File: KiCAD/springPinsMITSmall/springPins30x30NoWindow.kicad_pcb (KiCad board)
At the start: 2 copper layers, 30 x 30 mm, 22 parts, among them J1 CONN_02X06, J2 CONN_02X06

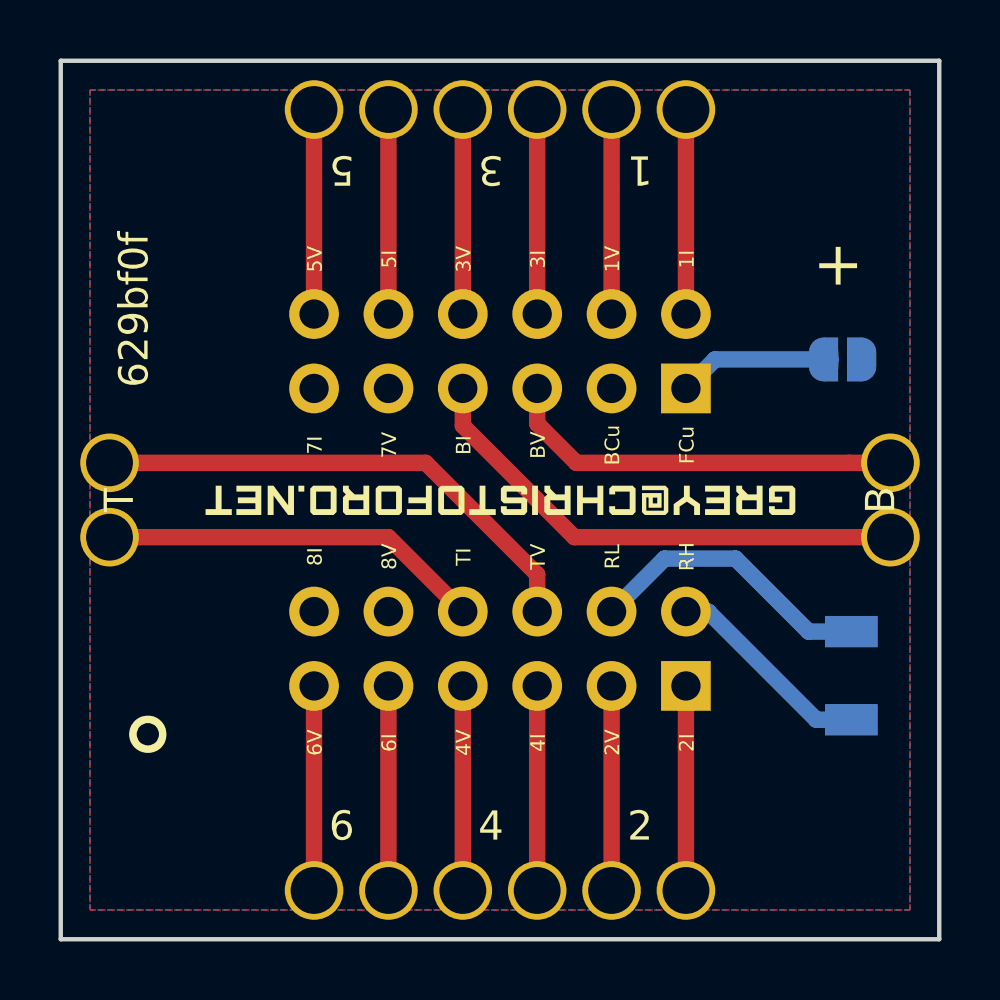
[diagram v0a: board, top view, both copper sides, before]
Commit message: update kicad and add logos
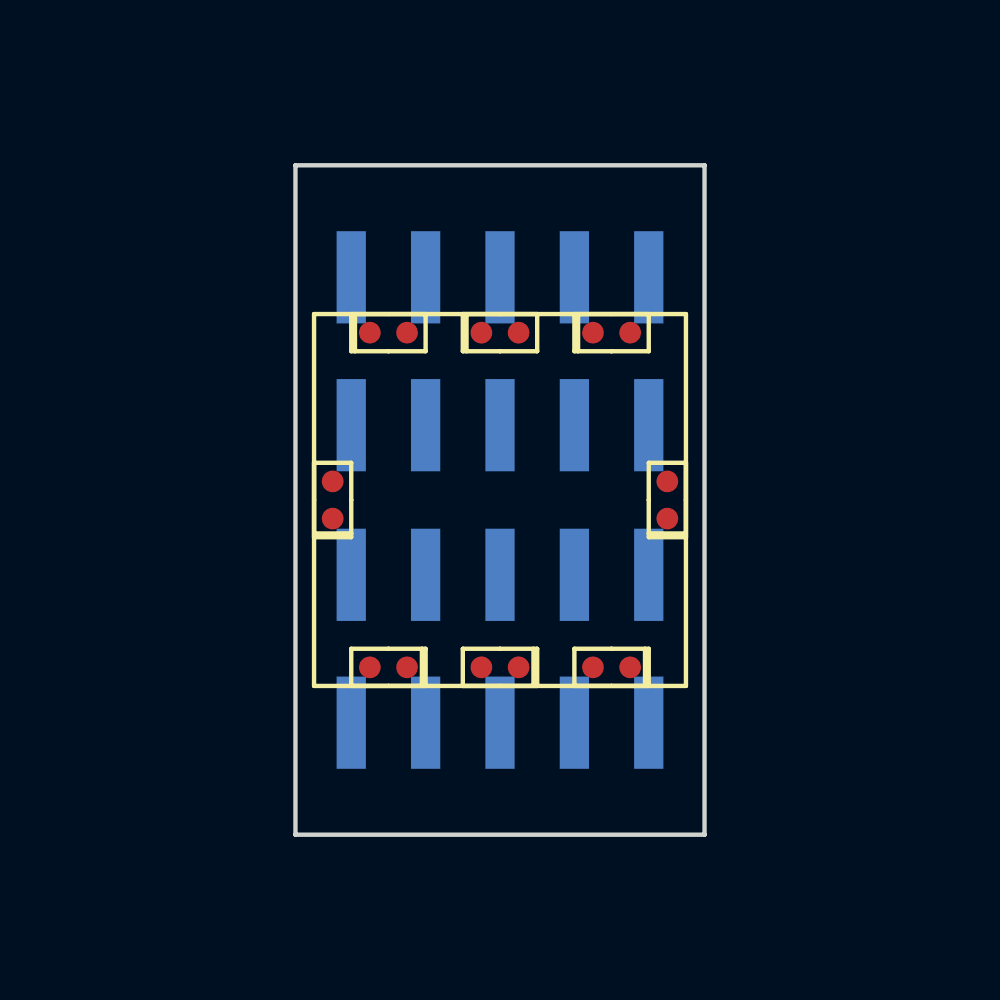
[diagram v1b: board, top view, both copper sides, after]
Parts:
- removed JP1: Jumper_NO_Small, Jumper:SolderJumper-2_P1.3mm_Open_RoundedPad1.0x1.5mm
- removed L1 (x2): GREY@CHRISTOFORO.NET, myParts:logo_small
- removed R1: 200k, Resistor_SMD:R_1206_3216Metric
- removed TP10, TP11, TP12, TP15, TP16, TP17, TP18, TP19, TP20, TP3, TP4, TP5, TP6, TP7, TP8, TP9: TEST, myParts:S25-022+P25-4023
- added REF**: 854-22-002-30-001101, myParts:854-22-002-30-001101, F.Cu at (-3.17, 5.71)
- added REF**: 854-22-002-30-001101, myParts:854-22-002-30-001101, F.Cu at (0.64, 5.71)
- added REF**: 854-22-002-30-001101, myParts:854-22-002-30-001101, F.Cu at (4.45, 5.71)
- added REF**: 854-22-002-30-001101, myParts:854-22-002-30-001101, F.Cu at (5.71, 0.64)
- added REF**: 854-22-002-30-001101, myParts:854-22-002-30-001101, F.Cu at (-5.71, 0.64)
- added REF**: 854-22-002-30-001101, myParts:854-22-002-30-001101, F.Cu at (-4.45, -5.71)
- added REF**: 854-22-002-30-001101, myParts:854-22-002-30-001101, F.Cu at (3.17, -5.71)
- added REF**: 854-22-002-30-001101, myParts:854-22-002-30-001101, F.Cu at (-0.64, -5.71)
- J1, J2: footprint Connector_PinHeader_2.54mm:PinHeader_2x06_P2.54mm_Vertical -> Connector_PinHeader_2.54mm:PinHeader_2x05_P2.54mm_Vertical_SMD
- moved J1 6.48 mm to (0.00, 5.08)
- moved J2 6.48 mm to (0.00, -5.08)
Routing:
- net /VT: track 17.5 -> 0.00 mm
- net /IB: track 17.5 -> 0.00 mm
- net /VB: track 13.8 -> 0.00 mm
- net /IT: track 13.1 -> 0.00 mm
- net /RL: track 9.97 -> 0.00 mm
- net /RH: track 7.18 -> 0.00 mm
- net /V6: track 6.99 -> 0.00 mm
- net /V5: track 6.99 -> 0.00 mm
- net /V4: track 6.99 -> 0.00 mm
- net /V3: track 6.99 -> 0.00 mm
- net /V2: track 6.99 -> 0.00 mm
- net /V1: track 6.99 -> 0.00 mm
- net /I6: track 6.99 -> 0.00 mm
- net /I5: track 6.99 -> 0.00 mm
- net /I4: track 6.99 -> 0.00 mm
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- removed copper zone on B.Cu, net /BCu
- removed copper zone on F.Cu, net /FCu
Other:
- board size 30 x 30 mm -> 14 x 22.9 mm
- board text removed: "+"
- board text removed: "1"
- board text removed: "2"
- board text removed: "3"
- board text removed: "4"
- board text removed: "5"
- board text removed: "6"
- board text removed: "629bf0f"
- board text removed: "B"
- board text removed: "T"
- board text removed: "°"
